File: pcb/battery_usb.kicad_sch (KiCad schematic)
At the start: 23 parts, among them SW1 SW_DIP_x01, U2 USB2514-HZH (C184347), U3 TPS62140, Y1 48mhz

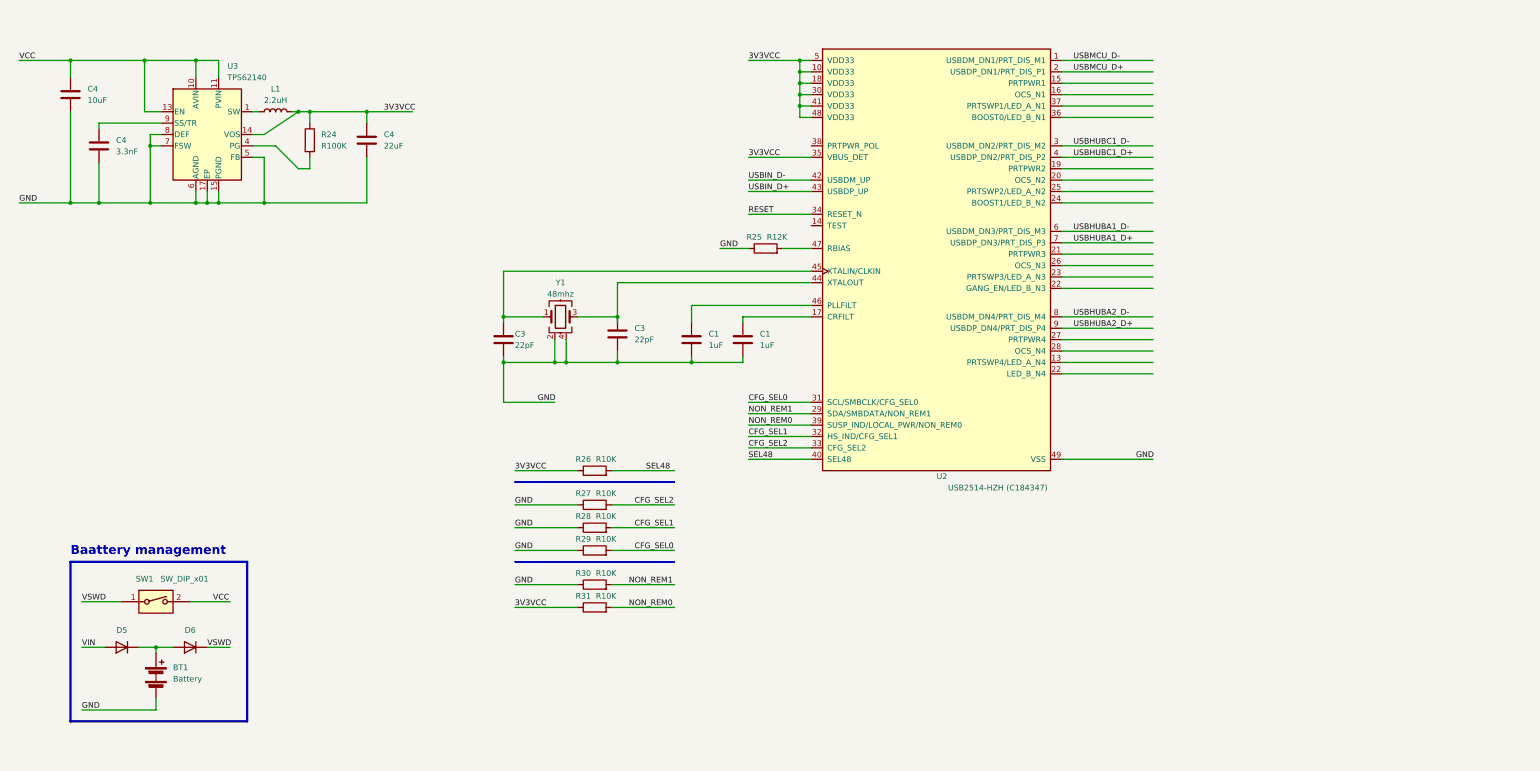
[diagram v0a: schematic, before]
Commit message: Implement USB Hub
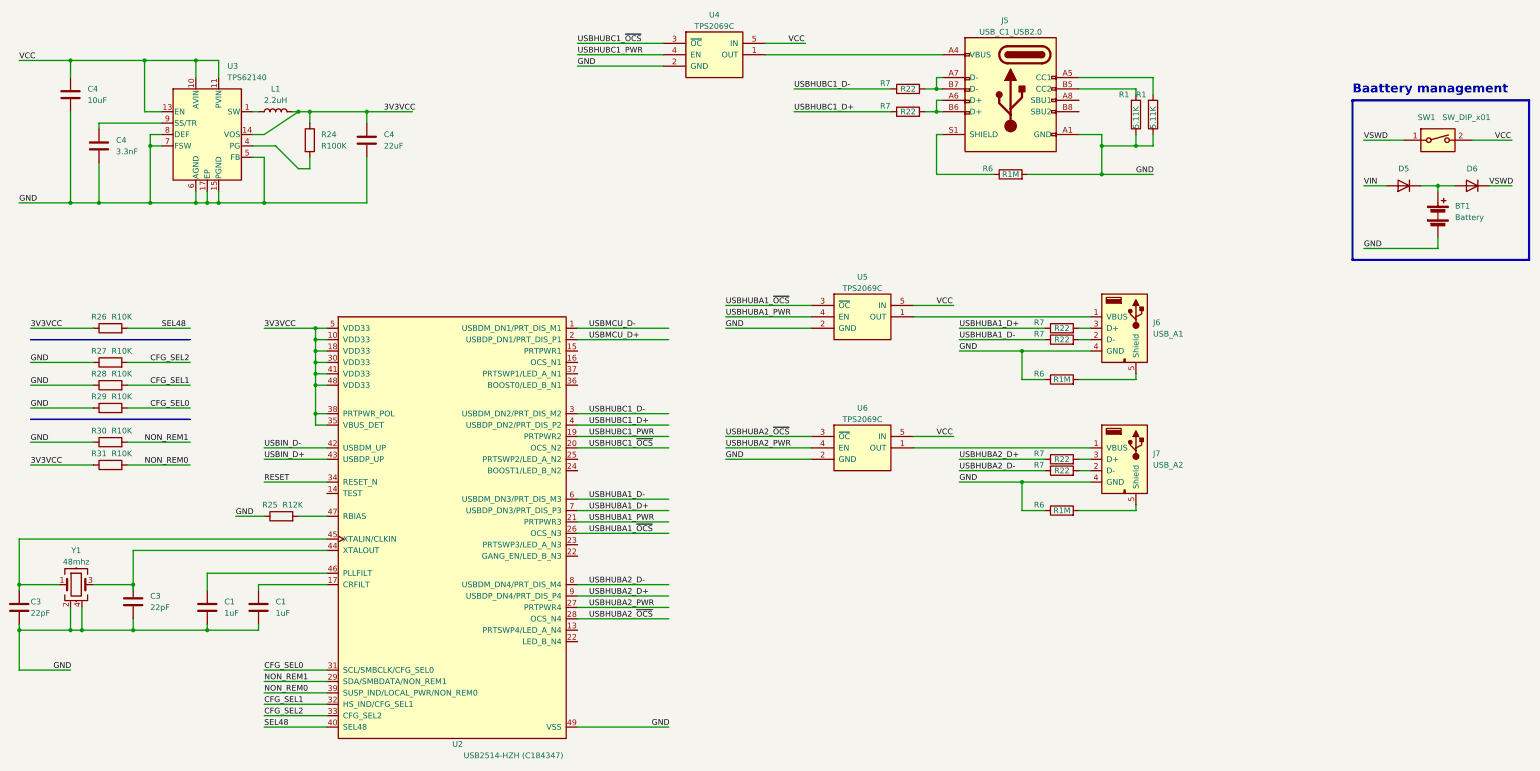
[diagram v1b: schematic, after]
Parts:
- added J5: USB_C1_USB2.0, Connector_USB:USB_C_Receptacle_G-Switch_GT-USB-7010ASV, symbol Connector:USB_C_Receptacle_USB2.0
- added J6: USB_A1, symbol Connector:USB_A
- added J7: USB_A2, symbol Connector:USB_A
- added R1 (x2): 5.11K, Resistor_SMD:R_0402_1005Metric, symbol Device:R
- added R6 (x3): R1M, Resistor_SMD:R_0603_1608Metric, symbol Device:R
- added R7 (x6): R22, Resistor_SMD:R_0402_1005Metric, symbol Device:R
- added U4, U5, U6: TPS2069C, Package_TO_SOT_SMD:SOT-23-5, symbol Power_Management:TPS2041B
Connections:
- net 3V3VCC: now also U2.38 (PRTPWR_POL)
- net GND: now also J5.A1 (GND), J5.A12 (GND), J5.B1 (GND), J5.B12 (GND), J6.4 (GND), J7.4 (GND), R1.2, R1.2, R6.1, R6.1, R6.2, U4.2 (GND), U5.2 (GND), U6.2 (GND)
- net USBHUBA1_D+: now also R7.1
- net USBHUBA1_D-: now also R7.1
- net USBHUBA2_D+: now also R7.1
- net USBHUBA2_D-: now also R7.1
- net USBHUBC1_D+: now also R7.1
- net USBHUBC1_D-: now also R7.1
- net VCC: now also U4.5 (IN), U5.5 (IN), U6.5 (IN)
- net USBHUBC1_PWR: now reaches U2.19 (PRTPWR2)
- net USBHUBC1_PWR: now also U4.4 (EN)
- net USBHUBC1_~{OCS}: now reaches U2.20 (OCS_N2)
- net USBHUBC1_~{OCS}: now also U4.3 (~{OC})
- net USBHUBA1_PWR: now reaches U2.21 (PRTPWR3)
- net USBHUBA1_PWR: now also U5.4 (EN)
- net USBHUBA1_~{OCS}: now reaches U2.26 (OCS_N3)
- net USBHUBA1_~{OCS}: now also U5.3 (~{OC})
- net USBHUBA2_PWR: now reaches U2.27 (PRTPWR4)
- net USBHUBA2_PWR: now also U6.4 (EN)
- net USBHUBA2_~{OCS}: now reaches U2.28 (OCS_N4)
- net USBHUBA2_~{OCS}: now also U6.3 (~{OC})
- new net: J5.A5 (CC1), R1.1
- new net: J6.1 (VBUS), U5.1 (OUT)
- new net: J5.B5 (CC2), R1.1
- new net: J5.A6 (D+), J5.B6 (D+), R7.2
- new net: J7.2 (D-), R7.2
- new net: J5.A4 (VBUS), J5.A9 (VBUS), J5.B4 (VBUS), J5.B9 (VBUS), U4.1 (OUT)
- new net: J5.A7 (D-), J5.B7 (D-), R7.2
- new net: J5.S1 (SHIELD), R6.1
- new net: J7.5 (Shield), R6.2
- new net: J7.3 (D+), R7.2
- new net: J7.1 (VBUS), U6.1 (OUT)
- new net: J6.2 (D-), R7.2
- new net: J6.3 (D+), R7.2
- new net: J6.5 (Shield), R6.2
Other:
- moved on the sheet: BT1, C1, C3, D5, D6, R25, R26, R27, R28, R29, R30, R31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
